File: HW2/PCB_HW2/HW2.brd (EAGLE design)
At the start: 50 x 49 mm, 22 parts

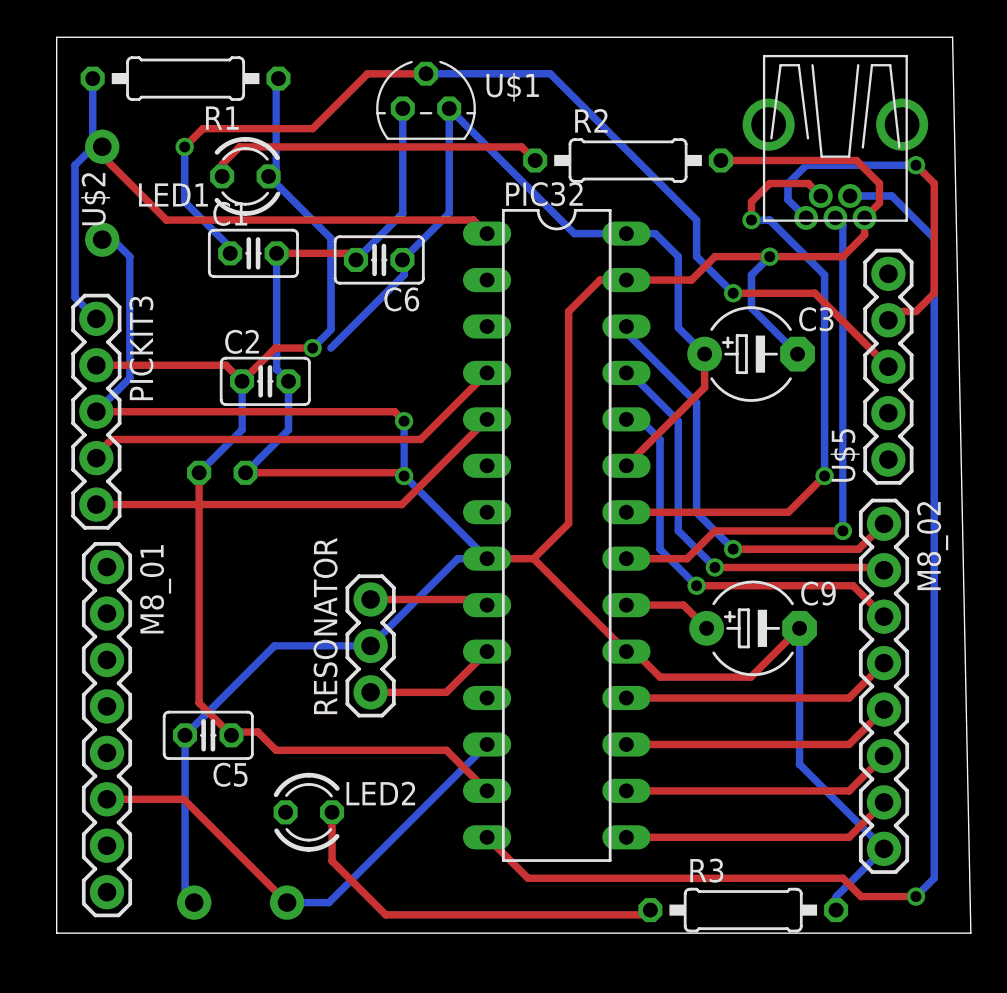
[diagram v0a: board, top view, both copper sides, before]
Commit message: Ready to be checked before order
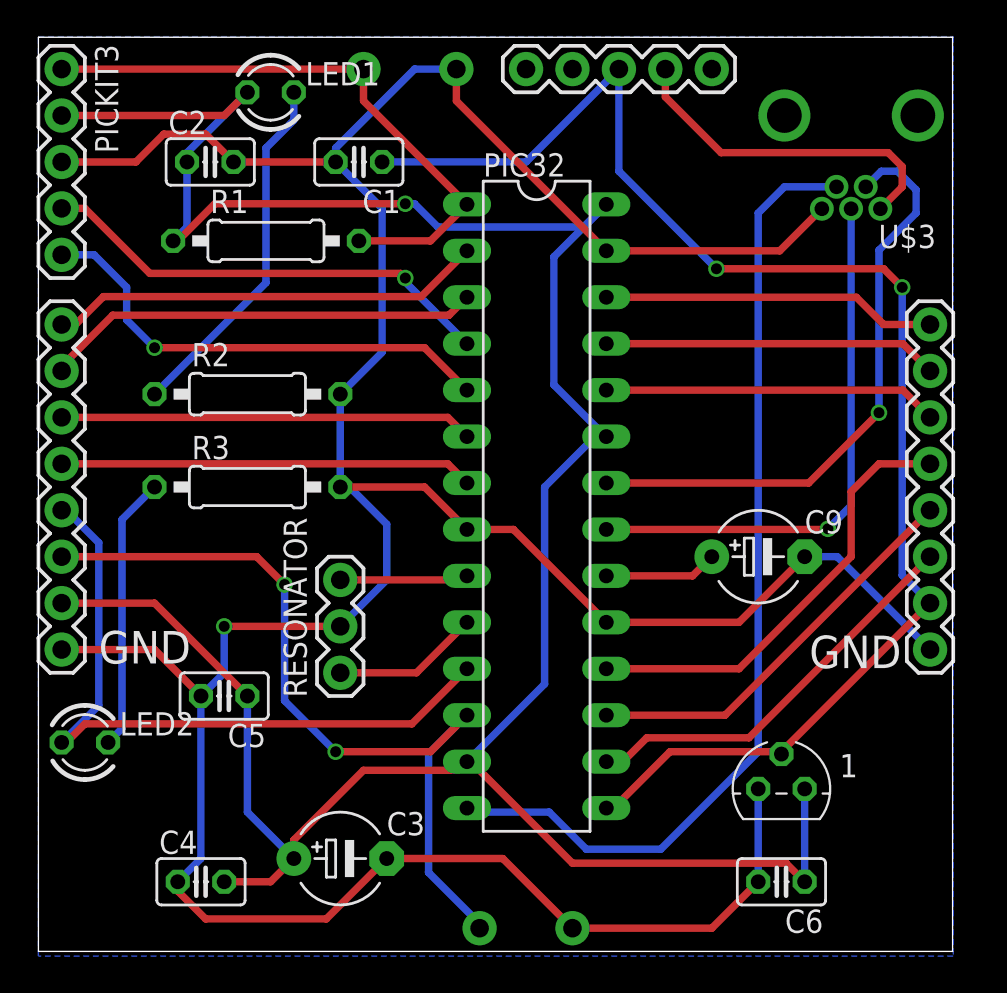
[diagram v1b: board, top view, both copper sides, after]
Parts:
- removed U$1: MCP1702, HWlib:TO92
- added 1: MCP1702, HWlib:TO92
- moved C6 40.5 mm to (40.6, 3.81)
- moved R3 35.7 mm to (11.4, 25.4)
- moved C3 35.6 mm to (16.5, 5.08)
- moved U$5 29.1 mm to (26.7, 48.3), turned to 0 degrees
- moved R2 24.4 mm to (11.4, 30.5)
- moved C4 22.4 mm to (8.89, 3.81), flipped to the top
- moved U$2 21.5 mm to (22.9, 48.3), turned to 180 degrees
- moved PICKIT3 13.8 mm to (1.27, 48.3)
- moved M8_01 13.5 mm to (1.27, 34.3)
- moved LED2 12.8 mm to (2.54, 11.4)
- moved C2 12.4 mm to (9.40, 43.2)
- moved M8_02 11.2 mm to (48.8, 34.3)
- moved U$4 10.6 mm to (24.1, 1.27), flipped to the top
- moved R1 9.91 mm to (12.4, 38.9), turned to 0 degrees
- moved C1 7.63 mm to (17.5, 43.2), turned to 180 degrees
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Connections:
- net +3V3: now also 1.3; no longer U$1.3
- net +5V: now also 1.2; no longer U$1.2
- net GND: now also 1.1; no longer U$1.1
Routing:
- net N$13: track 0.00 -> 38.4 mm
- net +3V3: track 112.6 -> 147.5 mm
- net N$11: track 0.00 -> 24.0 mm
- net N$9: track 0.00 -> 23.8 mm
- net N$17: track 0.00 -> 22.6 mm
- net N$15: track 0.00 -> 22.6 mm
- net N$16: track 26.7 -> 44.8 mm, vias 0 -> 2
- net N$4: track 66.8 -> 53.4 mm, vias 1 -> 0
- net N$22: track 14.9 -> 24.4 mm
- net +5V: track 69.7 -> 79.2 mm
- net N$26: track 14.9 -> 22.4 mm
- net N$23: track 14.9 -> 22.4 mm
- net N$14: track 21.4 -> 15.0 mm
- net N$19: track 23.4 -> 18.3 mm, vias 1 -> 0
- net N$2: track 38.0 -> 33.0 mm
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- added copper zone on layer 16, net GND
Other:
- board size 50 x 49 mm -> 50 x 50 mm
- board text added: "GND"
